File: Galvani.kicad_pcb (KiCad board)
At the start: 4 copper layers, 0 parts

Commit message: layout complete
Signed-off-by: Sean Cross <sean@xobs.io>
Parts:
- added AE1: PCB Antenna, RF_Antenna:Texas_SWRA117D_2.4GHz_Right, F.Cu at (115.4, 171.4)
- added C1: 10mF, Galvani:CAP-SMD_BD16.0-L17.0-W17.0-FD, F.Cu at (82.6, 164.0)
- added C10: Cap 1uF 0402, Capacitor_SMD:C_0402_1005Metric, F.Cu at (119.5, 157.5)
- added C11: Cap 100nF 0402, Capacitor_SMD:C_0402_1005Metric, F.Cu at (112.1, 163.9)
- added C12: Cap 10uF 0603, Capacitor_SMD:C_0603_1608Metric, F.Cu at (116.7, 165.3)
- added C13: Cap 10nF 0402, Capacitor_SMD:C_0402_1005Metric, F.Cu at (113.1, 163.5)
- added C14: Cap 100nF 0402, Capacitor_SMD:C_0402_1005Metric, F.Cu at (122.8, 151.8)
- added C15: Cap 100nF 0402, Capacitor_SMD:C_0402_1005Metric, F.Cu at (83.0, 151.6)
- added C16: Cap 100nF 0402, Capacitor_SMD:C_0402_1005Metric, F.Cu at (88.8, 151.6)
- added C17: 22uF, Capacitor_SMD:C_0805_2012Metric, F.Cu at (98.5, 151.4)
- added C18: Cap 22uF 0808, Capacitor_SMD:C_0805_2012Metric, F.Cu at (101.5, 145.0)
- added C19: Cap 12pF 0402, Capacitor_SMD:C_0402_1005Metric, F.Cu at (96.8, 163.0)
- added C2: 10mF, Galvani:CAP-SMD_BD16.0-L17.0-W17.0-FD, F.Cu at (65.4, 164.0)
- added C22: Cap 100nF 0402, Capacitor_SMD:C_0402_1005Metric, F.Cu at (53.6, 158.6)
- added C23: Cap 100nF 0402, Capacitor_SMD:C_0402_1005Metric, F.Cu at (57.7, 144.3)
- added C24: Cap 100nF 0402, Capacitor_SMD:C_0402_1005Metric, F.Cu at (92.0, 144.2)
- added C25: Cap 100nF 0402, Capacitor_SMD:C_0402_1005Metric, F.Cu at (125.1, 143.9)
- added C26: Cap 100nF 0402, Capacitor_SMD:C_0402_1005Metric, F.Cu at (135.9, 158.2)
- added C27: Cap 100nF 0402, Capacitor_SMD:C_0402_1005Metric, F.Cu at (124.6, 173.3)
- added C28: Cap 100nF 0402, Capacitor_SMD:C_0402_1005Metric, F.Cu at (92.1, 173.4)
- added C29: Cap 100nF 0402, Capacitor_SMD:C_0402_1005Metric, F.Cu at (56.6, 172.4)
- added C3: Cap 12pF 0402, Capacitor_SMD:C_0402_1005Metric, F.Cu at (102.3, 148.2)
- added C4: Cap 22uF 0808, Capacitor_SMD:C_0805_2012Metric, F.Cu at (99.0, 162.0)
- added C6: Cap 12pF 0201, Capacitor_SMD:C_0201_0603Metric, F.Cu at (109.9, 163.3)
- added C7: Cap 12pF 0201, Capacitor_SMD:C_0201_0603Metric, F.Cu at (109.9, 159.7)
- added C8: Cap 1uF 0402, Capacitor_SMD:C_0402_1005Metric, F.Cu at (119.1, 164.9)
- added C9: Cap 1uF 0402, Capacitor_SMD:C_0402_1005Metric, F.Cu at (120.5, 162.9)
- added CONN1: 2060-453/998-404, Galvani:CONN-SMD_2060-453, F.Cu at (144.1, 170.6)
- added CONN2: Bare Wire, Galvani:CONN-SMD_2060-453, F.Cu at (46.6, 170.4)
- added CONN3: 2060-453/998-404, Galvani:CONN-SMD_2060-453, F.Cu at (143.7, 147.0)
- added CONN4: 2060-453/998-404, Galvani:CONN-SMD_2060-453, F.Cu at (46.2, 146.2)
- added D1: DB207S, Galvani:DB-S_L8.3-W6.4-P5.10-LS9.9-TL, F.Cu at (58.3, 149.1)
- added D10: SS34, Diode_SMD:D_SMA, F.Cu at (104.0, 158.4)
- added D11: SS34, Diode_SMD:D_SMA, F.Cu at (104.0, 162.0)
- added D2: WS2812C-2020, Galvani:LED_WS2812B-2020_PLCC4_2.0x2.0mm, F.Cu at (58.3, 142.5)
- added D3: WS2812C-2020, Galvani:LED_WS2812B-2020_PLCC4_2.0x2.0mm, F.Cu at (51.8, 158.0)
- added D4: WS2812C-2020, Galvani:LED_WS2812B-2020_PLCC4_2.0x2.0mm, F.Cu at (92.4, 142.4)
- added D5: WS2812C-2020, Galvani:LED_WS2812B-2020_PLCC4_2.0x2.0mm, F.Cu at (125.7, 142.2)
- added D6: WS2812C-2020, Galvani:LED_WS2812B-2020_PLCC4_2.0x2.0mm, F.Cu at (137.8, 158.8)
- added D7: WS2812C-2020, Galvani:LED_WS2812B-2020_PLCC4_2.0x2.0mm, F.Cu at (124.0, 175.1)
- added D8: WS2812C-2020, Galvani:LED_WS2812B-2020_PLCC4_2.0x2.0mm, F.Cu at (91.5, 175.3)
- added D9: WS2812C-2020, Galvani:LED_WS2812B-2020_PLCC4_2.0x2.0mm, F.Cu at (56.0, 174.2)
- added F1: SRF1206P150, Fuse:Fuse_1206_3216Metric, F.Cu at (101.6, 165.0)
- added J1: USB-C Receptacle, Galvani:USB-C-SMD_TYPE-C16PIN, F.Cu at (117.4, 145.1)
- added J2: U.FL Connector, Connector_Coaxial:U.FL_Hirose_U.FL-R-SMT-1_Vertical, F.Cu at (120.1, 169.5)
- added J3: JST-PH, Connector_JST:JST_PH_S3B-PH-SM4-TB_1x03-1MP_P2.00mm_Horizontal, F.Cu at (146.3, 158.8)
- added J4: JST-PH, Connector_JST:JST_PH_S3B-PH-SM4-TB_1x03-1MP_P2.00mm_Horizontal, F.Cu at (44.3, 158.2)
- added L1: 22uH, Galvani:IND-SMD_L7.1-W6.6, F.Cu at (95.5, 167.8)
- added L2: L 20nH 0201, Inductor_SMD:L_0201_0603Metric, F.Cu at (112.6, 162.1)
- added L3: 22uH, Galvani:IND-SMD_L7.1-W6.6, F.Cu at (106.9, 148.8)
- added P1: Cap 1.5pF 0201, Capacitor_SMD:C_0201_0603Metric, F.Cu at (115.7, 168.6)
- added P2: L 2.7 nH 0201, Inductor_SMD:L_0201_0603Metric, F.Cu at (115.3, 167.5)
- added P3: Cap 1.5pF 0201, Capacitor_SMD:C_0201_0603Metric, F.Cu at (115.7, 166.4)
- added R1: R 5.1k 0402, Resistor_SMD:R_0402_1005Metric, F.Cu at (123.2, 146.9)
- added R10: R 20k 0402, Resistor_SMD:R_0402_1005Metric, F.Cu at (81.2, 147.6)
- added R11: R 22.1k 0402, Resistor_SMD:R_0402_1005Metric, F.Cu at (97.9, 148.8)
- added R12: R 20k 0402, Resistor_SMD:R_0402_1005Metric, F.Cu at (81.2, 149.6)
- added R13: R 20k 0402, Resistor_SMD:R_0402_1005Metric, F.Cu at (86.8, 151.6)
- added R14: R 20k 0402, Resistor_SMD:R_0402_1005Metric, F.Cu at (84.9, 151.6)
- added R15: R 20k 0402, Resistor_SMD:R_0402_1005Metric, F.Cu at (97.9, 146.8)
- added R16: R 20k 0402, Resistor_SMD:R_0402_1005Metric, F.Cu at (115.3, 170.0)
- added R17: R 20k 0402, Resistor_SMD:R_0402_1005Metric, F.Cu at (115.8, 169.5)
- added R2: R 20k 0402, Resistor_SMD:R_0402_1005Metric, F.Cu at (97.2, 158.2)
- added R3: R 20k 0402, Resistor_SMD:R_0402_1005Metric, F.Cu at (95.2, 158.2)
- added R4: R 5.1k 0402, Resistor_SMD:R_0402_1005Metric, F.Cu at (111.6, 146.9)
- added R5: R 20k 0402, Resistor_SMD:R_0402_1005Metric, F.Cu at (132.2, 158.0)
- added R6: R 20k 0402, Resistor_SMD:R_0402_1005Metric, F.Cu at (121.1, 160.5)
- added R7: R 20k 0402, Resistor_SMD:R_0402_1005Metric, F.Cu at (132.0, 162.4)
- added R8: R 20k 0402, Resistor_SMD:R_0402_1005Metric, F.Cu at (117.8, 166.7)
- added R9: R 20k 0402, Resistor_SMD:R_0402_1005Metric, F.Cu at (121.5, 162.0)
- added SW1: Pushbutton 4.2x3.2mm 250gf, Button_Switch_SMD:SW_Push_1P1T_XKB_TS-1187A, F.Cu at (129.4, 154.6)
- added SW2: Pushbutton 4.2x3.2mm 250gf, Button_Switch_SMD:SW_Push_1P1T_XKB_TS-1187A, F.Cu at (129.2, 165.9)
- added U1: TPS560430, Package_TO_SOT_SMD:SOT-23-6, F.Cu at (95.8, 160.8)
- added U2: ESP32-C3FN4, Package_DFN_QFN:QFN-32-1EP_5x5mm_P0.5mm_EP3.45x3.45mm, F.Cu at (116.9, 161.3)
- added U3: W25Q128JVS, Package_SO:SOIC-8_5.23x5.23mm_P1.27mm, F.Cu at (117.2, 153.7)
- added U4: SN74LVC4245APWR, Galvani:TSSOP-24_L7.8-W4.4-P0.65-LS6.4-BL, F.Cu at (86.0, 146.9)
- added U5: TPS560430, Package_TO_SOT_SMD:SOT-23-6, F.Cu at (100.1, 148.2)
- added Y1: Crystal 40MHz 2016, Galvani:Crystal_SMD_2016-4Pin_2.0x1.6mm, F.Cu at (110.5, 161.5)
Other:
- board outline added: 114.3 x 38.1 mm

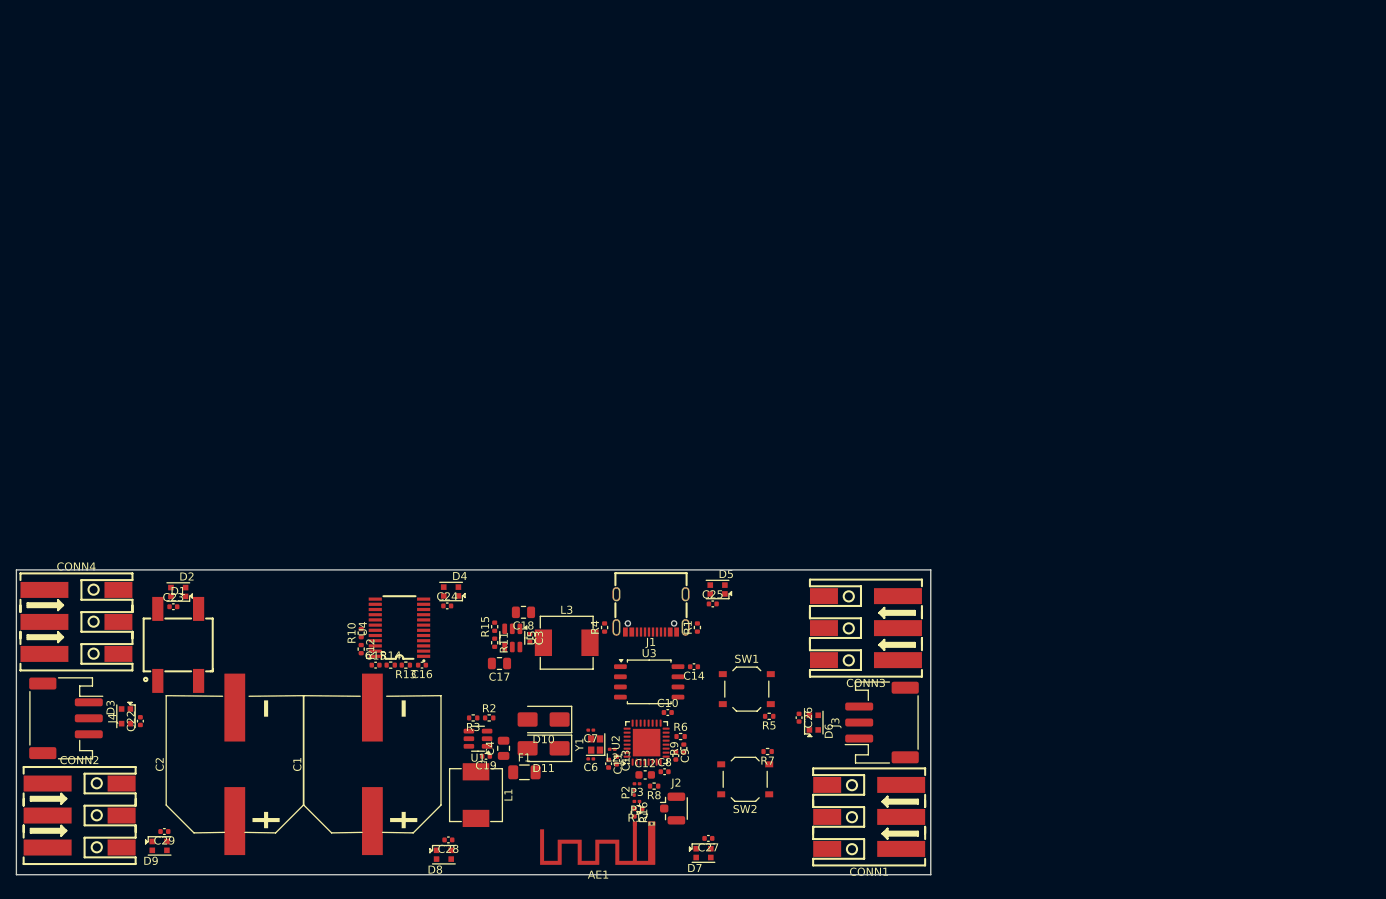
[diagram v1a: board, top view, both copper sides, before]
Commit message: evt1: initial release
Signed-off-by: Sean Cross <sean@xobs.io>
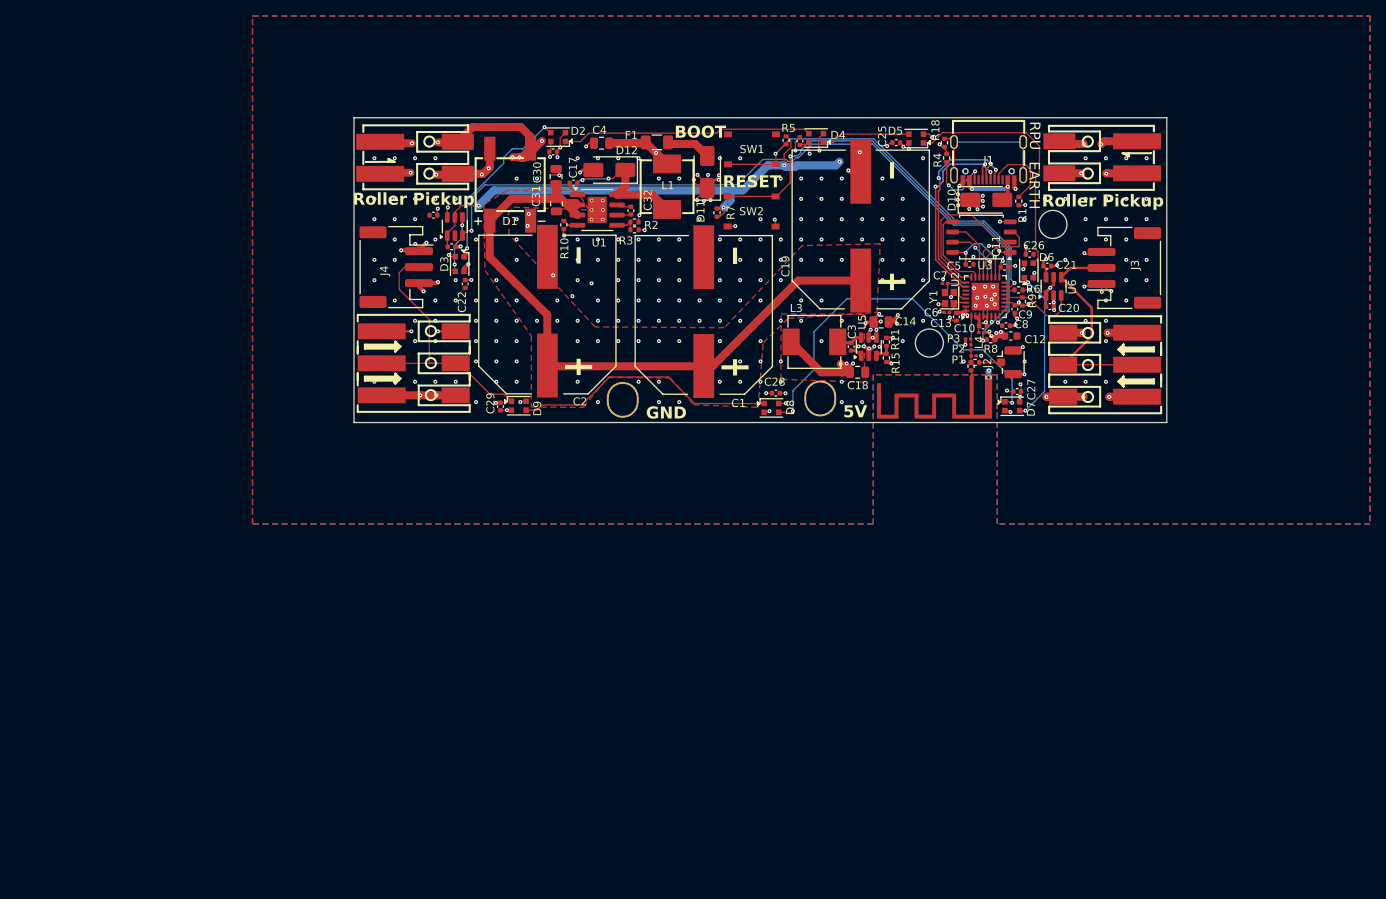
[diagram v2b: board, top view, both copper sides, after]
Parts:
- removed L2: L 20nH 0201, Inductor_SMD:L_0201_0603Metric
- removed R12, R13, R14: R 20k 0402, Resistor_SMD:R_0402_1005Metric
- added C20: Cap 100nF 0402, Capacitor_SMD:C_0402_1005Metric, F.Cu at (167.3, 106.8)
- added C21: Cap 100nF 0402, Capacitor_SMD:C_0402_1005Metric, F.Cu at (167.0, 101.7)
- added C30: Cap 10uF 0805, Capacitor_SMD:C_0805_2012Metric, F.Cu at (105.6, 90.5)
- added C31: Cap 10uF 0805, Capacitor_SMD:C_0805_2012Metric, F.Cu at (105.6, 93.9)
- added C32: Cap 10nF 0402, Capacitor_SMD:C_0402_1005Metric, F.Cu at (114.9, 94.8)
- added C5: Cap 100nF 0402, Capacitor_SMD:C_0402_1005Metric, F.Cu at (157.2, 101.5)
- added D12: SS34, Diode_SMD:D_SMA, F.Cu at (112.2, 89.7)
- added H2: Mounting Hole, MountingHole:MountingHole_3.5mm, F.Cu at (152.2, 111.3)
- added H3: Mounting Hole, MountingHole:MountingHole_3.5mm, F.Cu at (167.7, 96.5)
- added L4: L 2.7 nH 0201, Inductor_SMD:L_0201_0603Metric, F.Cu at (158.7, 110.0)
- added R18: R 20k 0402, Resistor_SMD:R_0402_1005Metric, F.Cu at (154.1, 86.3)
- added TP1: GND, Galvani:Test Point, F.Cu at (113.9, 118.4)
- added TP2: 5V, Galvani:Test Point, F.Cu at (138.6, 118.3)
- added U6: SN74LVC1T45DBVR, Package_TO_SOT_SMD:SOT-23-6, F.Cu at (167.8, 104.3)
- added kibuzzard-66F0D9A1: G***, kibuzzard-66F0D9A1, B.Cu at (129.7, 93.2)
- added kibuzzard-66F0D9BF: G***, kibuzzard-66F0D9BF, B.Cu at (141.9, 96.5)
- C1, C2: value 10mF -> 1.8mF; footprint Galvani:CAP-SMD_BD16.0-L17.0-W17.0-FD -> Galvani:CAP-SMD_BD18.0-L21.5-W21.5
- C14: value Cap 100nF 0402 -> Cap 22uF 0805; footprint Capacitor_SMD:C_0402_1005Metric -> Capacitor_SMD:C_0805_2012Metric
- C17: value 22uF -> Cap 100nF 0402; footprint Capacitor_SMD:C_0805_2012Metric -> Capacitor_SMD:C_0402_1005Metric
- C18, C4: value Cap 22uF 0808 -> Cap 22uF 0805
- C19: value Cap 12pF 0402 -> 1.8mF; footprint Capacitor_SMD:C_0402_1005Metric -> Galvani:CAP-SMD_BD18.0-L21.5-W21.5
- C3: value Cap 12pF 0402 -> Cap 100nF 0402
- CONN1: value 2060-453/998-404 -> Bare Wire
- CONN3, CONN4: value 2060-453/998-404 -> Wire Connector; footprint Galvani:CONN-SMD_2060-453 -> Galvani:CONN-SMD_2060-452
- D1: value DB207S -> DB307S
- L1: value 22uH -> 4.7uH; footprint Galvani:IND-SMD_L7.1-W6.6 -> Galvani:IND-SMD_L7.2-W6.6_GPSR07X0
- U1: value TPS560430 -> LMR14030SDDAR; footprint Package_TO_SOT_SMD:SOT-23-6 -> Package_SO:SOIC-8-1EP_3.9x4.9mm_P1.27mm_EP2.41x3.3mm_ThermalVias
- U4: value SN74LVC4245APWR -> SN74LVC1T45DBVR; footprint Galvani:TSSOP-24_L7.8-W4.4-P0.65-LS6.4-BL -> Package_TO_SOT_SMD:SOT-23-6
- moved D10 85.3 mm to (159.3, 93.4), turned to 0 degrees
- moved C19 81.2 mm to (143.6, 96.7), turned to 90 degrees
- moved F1 80.5 mm to (118.2, 86.3)
- moved L1 79.7 mm to (119.4, 91.8), turned to 90 degrees
- moved C11 79.4 mm to (161.6, 101.8), turned to 0 degrees
- moved C4 76.6 mm to (111.3, 86.4), turned to 180 degrees
- moved D11 74.9 mm to (124.5, 90.0), turned to 90 degrees
- moved C23 74.1 mm to (105.2, 87.4)
- moved D2 74.1 mm to (105.8, 85.6)
- moved C24 72.9 mm to (136.0, 86.1), turned to 90 degrees
- moved D4 72.8 mm to (138.1, 85.7)
- moved R4 72.6 mm to (154.4, 88.2)
- moved R5 72.0 mm to (134.3, 86.0), turned to -90 degrees
- moved CONN4 71.7 mm to (88.4, 88.2)
- moved C12 71.4 mm to (162.4, 110.5)
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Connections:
- C10 pad 1: VWIFI -> Net-(C10-Pad1)
- C14 pad 1: GND -> V5V
- C14 pad 2: VSPI -> GND
- C17 pad 1: V5V -> Net-(D12-K)
- C17 pad 2: GND -> Net-(U1-BOOT)
- C19 pad 1: Net-(U1-CB) -> /VAC_RECTIFIED
- C19 pad 2: Net-(U1-SW) -> GND
- C3 pad 1: Net-(U5-CB) -> Net-(U5-SW)
- C3 pad 2: Net-(U5-SW) -> Net-(U5-CB)
- C6 pad 1: Net-(C6-Pad1) -> Net-(U2-XTAL_P)
- CONN1 pad 1: GND -> V5V
- CONN1 pad 3: V5V -> GND
- CONN2 pad 1: GND -> V5V
- CONN2 pad 3: V5V -> GND
- CONN3 pad 2: unconnected-(CONN3-Pad2) -> VAC
- CONN4 pad 2: unconnected-(CONN4-Pad2)_1 -> Earth
- J1 pad 1: (no net) -> Net-(J1-Shell-Pad1)
- J1 pad 2: (no net) -> Net-(J1-Shell-Pad1)
- J1 pad 3: (no net) -> Net-(J1-Shell-Pad1)
- J1 pad 4: (no net) -> Net-(J1-Shell-Pad1)
- J3 pad MP: (no net) -> GND
- J4 pad MP: (no net) -> GND
- L1 pad 1: Net-(U1-SW) -> Net-(D12-K)
- R10 pad 1: Net-(U4-OE#) -> GND
- R10 pad 2: GND -> Net-(U1-RT/SYNC)
- U1 pad 1: Net-(U1-CB) -> Net-(U1-BOOT)
- U1 pad 2: GND -> /VAC_RECTIFIED
- U1 pad 3: Net-(U1-FB) -> /VAC_RECTIFIED
- U1 pad 4: /VAC_RECTIFIED -> Net-(U1-RT/SYNC)
- U1 pad 5: /VAC_RECTIFIED -> Net-(U1-FB)
- U1 pad 6: Net-(U1-SW) -> Net-(U1-SS)
- U2 pad 2: VWIFI -> Net-(C10-Pad1)
- U2 pad 3: VWIFI -> Net-(C10-Pad1)
- U2 pad 4: unconnected-(U2-XTAL_32K_P/ADC1_CH0-Pad4) -> GND
- U2 pad 5: unconnected-(U2-XTAL_32K_N/ADC1_CH1-Pad5) -> GND
- U4 pad 1: V5V -> VWIFI
- U4 pad 2: Net-(U4-DIR) -> GND
- U4 pad 3: /LED_INTERNAL_5V -> /LED_INTERNAL
- U4 pad 4: /LED_EXTERNAL_5V -> /LED_INTERNAL_5V
- U4 pad 5: unconnected-(U4-A3-Pad5) -> VWIFI
- U4 pad 6: unconnected-(U4-A4-Pad6) -> V5V
- Y1 pad 1: Net-(C6-Pad1) -> Net-(U2-XTAL_P)
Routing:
- net VWIFI: track 0.00 -> 190.4 mm, vias 0 -> 19
- net VAC: track 0.00 -> 123.3 mm, vias 0 -> 7
- net Earth: track 0.00 -> 110.2 mm, vias 0 -> 6
- net /LED_INTERNAL: track 0.00 -> 95.2 mm, vias 0 -> 3
- net /VAC_RECTIFIED: track 0.00 -> 81.2 mm
- net GND: track 0.00 -> 78.2 mm, vias 0 -> 289
- net V5V: track 0.00 -> 71.8 mm, vias 0 -> 50
- net /RESET: track 0.00 -> 60.3 mm, vias 0 -> 2
- net /BOOT_MODE: track 0.00 -> 50.8 mm, vias 0 -> 2
- net Net-(D7-DOUT): track 0.00 -> 47.4 mm, vias 0 -> 2
- net Net-(D9-DOUT): track 0.00 -> 34.1 mm
- net Net-(D8-DOUT): track 0.00 -> 32.8 mm
- net Net-(D2-DOUT): track 0.00 -> 31.3 mm
- net Net-(D5-DOUT): track 0.00 -> 30.6 mm
- net /LED_EXTERNAL_5V: track 0.00 -> 28.8 mm
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- added copper zone on F.Cu, net /VAC_RECTIFIED
- added copper zone on B.Cu, net GND
- added copper zone on F.Cu, net GND
- added copper zone on In1.Cu, net GND
- added copper zone on In2.Cu, net V5V
- added copper zone on F.Cu, net VWIFI
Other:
- board size 114.3 x 38.1 mm -> 101.6 x 38.1 mm
- board text added: "5V"
- board text added: "BOOT"
- board text added: "EARTH"
- board text added: "External"
- board text added: "G"
- board text added: "GND"
- board text added: "Onboard"
- board text added: "Onboard LEDs are connected to GPIO2 External LEDs are connected to GPIO6 Hold BOOT while pressing RESET to program"
- board text added: "RESET"
- board text added: "RPU"
- board text added: "Roller Pickup"
- board text added: "SIG"
- board text added: "Side Rail"
- board text added: "WARNING: 3A Maximum! Connect no more than 50 lights!"
